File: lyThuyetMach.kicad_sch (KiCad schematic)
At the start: 34 parts, among them J1 USB_C_Receptacle_PowerOnly_6P, J2 Voltage_Booster, J4 Out_LED, Q1 BC547, Q2 BC547, Q3 BC547, Q4 BC547, Q5 BC547, Q6 BC547, Q7 TIP122, SW1 SW_SPDT, SW2 SW_SPDT

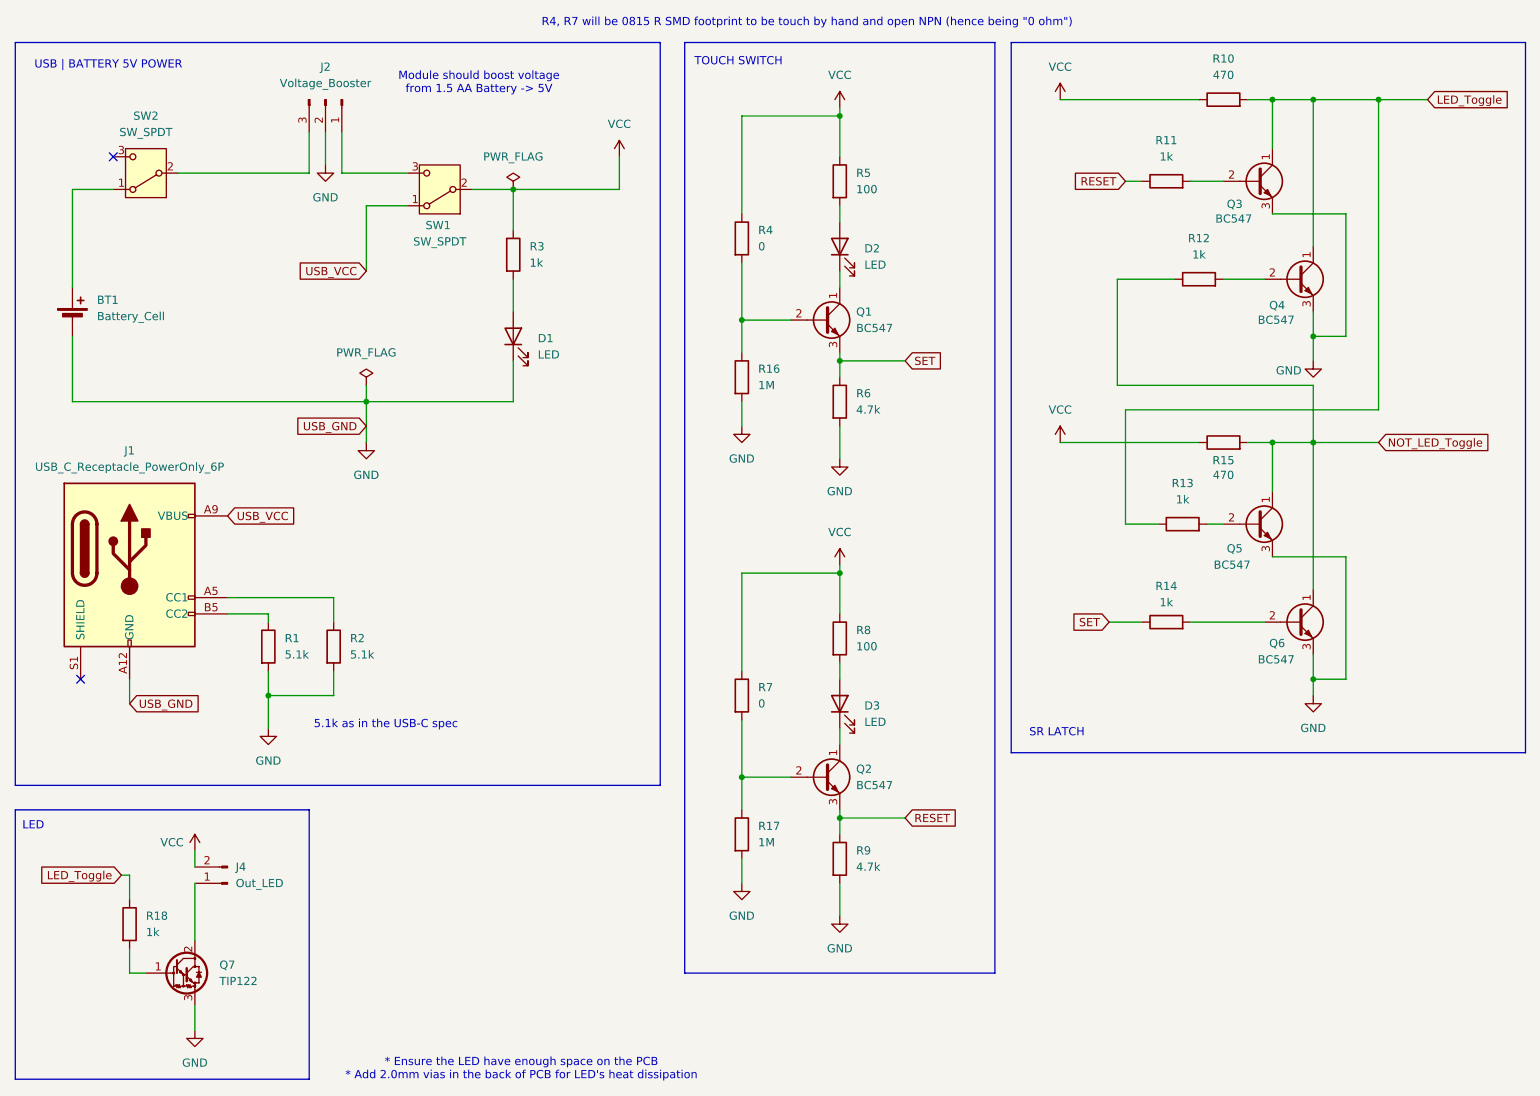
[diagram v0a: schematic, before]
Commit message: Add files via upload
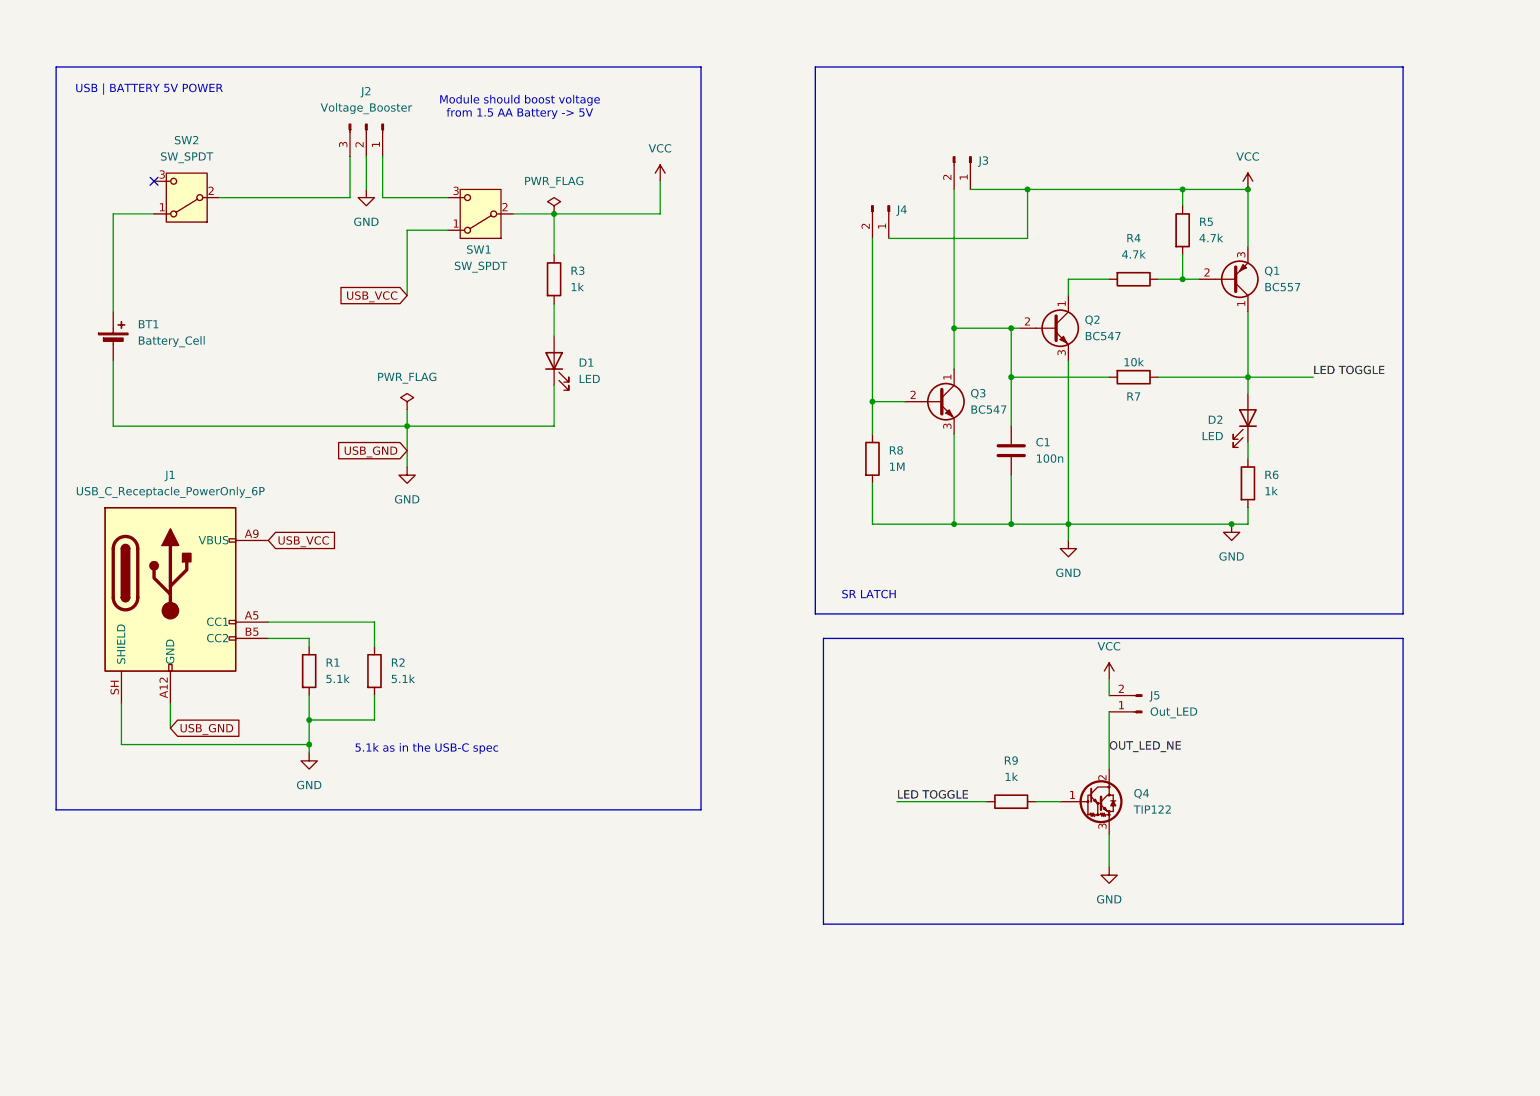
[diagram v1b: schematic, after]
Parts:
- removed D3: LED, LED_THT:LED_D5.0mm_FlatTop, symbol Device:LED
- removed Q1, Q4, Q5, Q6: BC547, Package_TO_SOT_THT:TO-92_Inline, symbol Transistor_BJT:BC547
- removed Q7: TIP122, Package_TO_SOT_THT:TO-220-3_Vertical, symbol Transistor_BJT:TIP122
- removed R10, R15: 470, Resistor_THT:R_Axial_DIN0207_L6.3mm_D2.5mm_P10.16mm_Horizontal, symbol Device:R
- removed R11, R12, R13, R14, R18: 1k, Resistor_THT:R_Axial_DIN0207_L6.3mm_D2.5mm_P10.16mm_Horizontal, symbol Device:R
- removed R16, R17: 1M, Resistor_THT:R_Axial_DIN0207_L6.3mm_D2.5mm_P10.16mm_Horizontal, symbol Device:R
- added C1: 100n, Capacitor_THT:C_Disc_D5.0mm_W2.5mm_P5.00mm, symbol Device:C
- added J3: Conn_01x02_Pin, Resistor_SMD:R_0815_2038Metric_Pad1.20x4.05mm_HandSolder, symbol Connector:Conn_01x02_Pin
- added J5: Out_LED, Connector_PinHeader_2.54mm:PinHeader_1x02_P2.54mm_Vertical, symbol Connector:Conn_01x02_Pin
- added Q1: BC557, Package_TO_SOT_THT:TO-92_Inline, symbol Transistor_BJT:BC557
- added Q4: TIP122, Package_TO_SOT_THT:TO-220-3_Vertical, symbol Transistor_BJT:TIP122
- D2: footprint LED_THT:LED_D5.0mm_FlatTop -> LED_THT:LED_D5.0mm
- J4: value Out_LED -> Conn_01x02_Pin; footprint Connector_PinHeader_2.54mm:PinHeader_1x02_P2.54mm_Vertical -> Resistor_SMD:R_0815_2038Metric_Pad1.20x4.05mm_HandSolder
- R4: value 0 -> 4.7k; footprint Resistor_SMD:R_0815_2038Metric_Pad1.20x4.05mm_HandSolder -> Resistor_THT:R_Axial_DIN0207_L6.3mm_D2.5mm_P10.16mm_Horizontal
- R5: value 100 -> 4.7k
- R6, R9: value 4.7k -> 1k
- R7: value 0 -> 10k; footprint Resistor_SMD:R_0815_2038Metric_Pad1.20x4.05mm_HandSolder -> Resistor_THT:R_Axial_DIN0207_L6.3mm_D2.5mm_P10.16mm_Horizontal
- R8: value 100 -> 1M
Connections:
- net LED_Toggle is gone; now on an unnamed net: Q3.1 (C)
- net SET is gone; now on an unnamed net: R6.1
- net GND: now also J1.SH (SHIELD), Q2.3 (E), R8.2, C1.2, Q4.3 (E); no longer R9.2
- net VCC: now also J4.1 (Pin_1), J3.1 (Pin_1), J5.2 (Pin_2), Q1.3 (E); no longer J4.2 (Pin_2), R4.1, R7.1, R8.1
- net at R4.2: now also Q2.1 (C)
- net at R5.2: now also R4.1, Q1.2 (B); no longer D2.2 (A)
- net at Q3.2 (B): now also J4.2 (Pin_2), R8.1
- net at Q2.2 (B), R7.2: now also C1.1, J3.2 (Pin_2)
- net RESET renamed LED TOGGLE
- net LED TOGGLE: now also D2.2 (A), R7.1, Q1.1 (C); no longer Q2.3 (E)
- new net: Q4.1 (B), R9.2
- new net OUT_LED_NE: J5.1 (Pin_1), Q4.2 (C)
- no-connect marks 2 -> 1
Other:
- note removed: "* Ensure the LED have enough space on the PCB * Add 2.0mm vias in the back of PCB for LED's heat dissipation"
- note removed: "LED"
- note removed: "R4, R7 will be 0815 R SMD footprint to be touch by hand and open NPN (hence being "0 ohm")"
- note removed: "TOUCH SWITCH"
- moved on the sheet: BT1, D1, J1, J2, R1, R2, R3, SW1, SW2
